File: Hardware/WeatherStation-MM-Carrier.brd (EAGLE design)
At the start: 67.3 x 58.4 mm, 156 parts, among them J11 microSD, J13 RJ11 - WIND, J15 MICROMOD-2222-C, J2 JTAG, J3 QWIIC_RIGHT_ANGLE, J7 RJ11 - RAIN, U1 BME280, U2 VEML6075, U3 AS3935, U5 AP7361C-33FGEUDFN-8

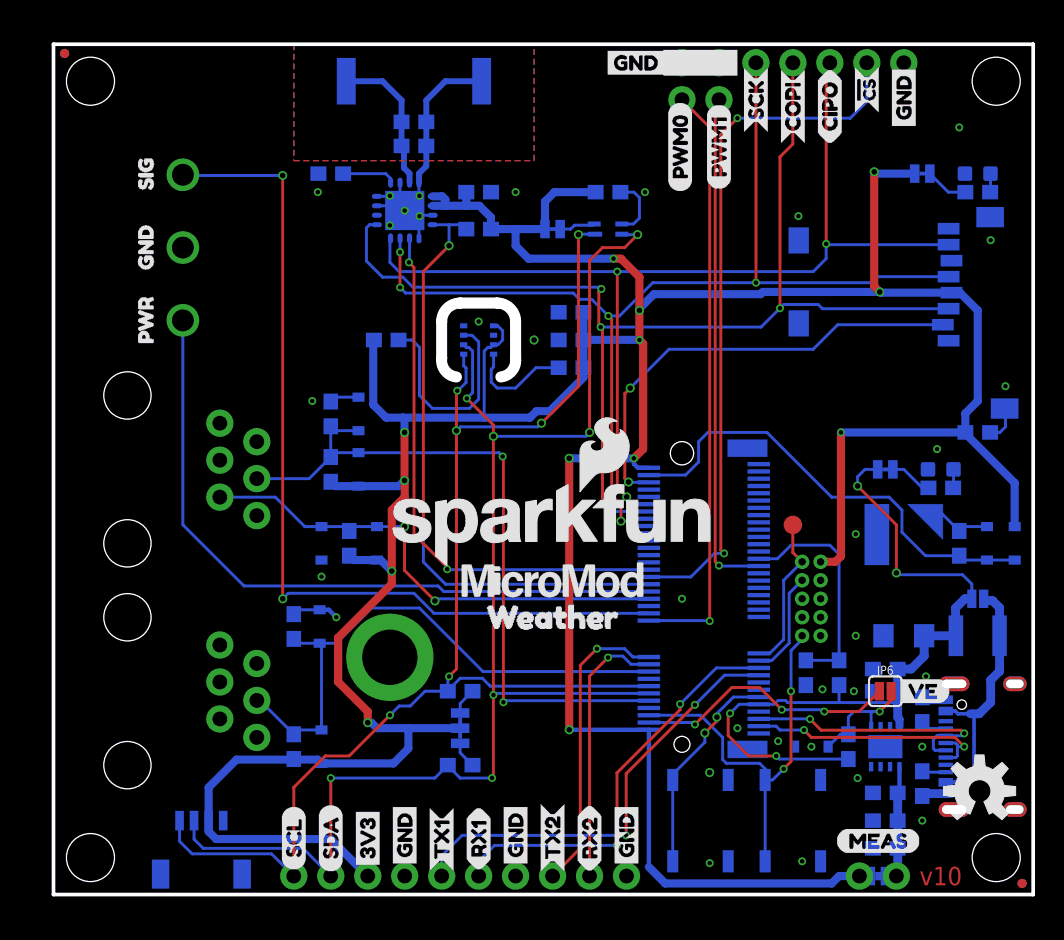
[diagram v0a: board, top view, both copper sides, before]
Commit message: Update WeatherStation-MM-Carrier.brd
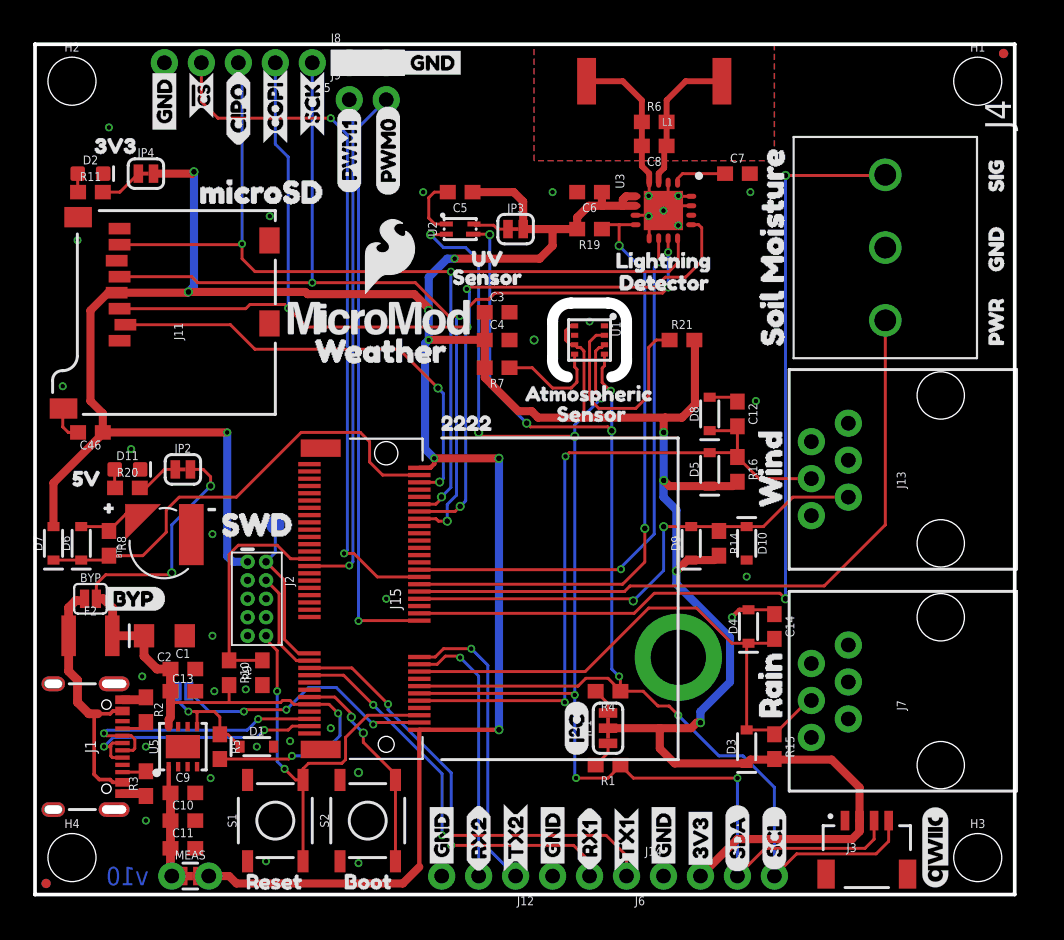
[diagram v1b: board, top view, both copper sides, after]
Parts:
- moved FD1 67.1 mm to (0.76, 0.76), flipped to the top
- moved FD3 67.1 mm to (0.76, 0.76), flipped to the bottom
- moved D7 66.0 mm to (1.27, 24.1), flipped to the top
- moved U$18 65.3 mm to (1.65, 28.6), flipped to the top
- moved FD2 64.5 mm to (66.5, 57.8), flipped to the top
- moved FD4 64.5 mm to (66.5, 57.8), flipped to the bottom
- moved H2 63.5 mm to (2.54, 55.9), flipped to the top
- moved H4 63.5 mm to (2.54, 2.54), flipped to the top
- moved U$12 63.5 mm to (66.0, 36.8), flipped to the top
- moved U$13 63.5 mm to (66.0, 47.4), flipped to the top
- moved U$4 63.5 mm to (66.0, 41.9), flipped to the top
- moved D6 62.2 mm to (3.17, 24.1), flipped to the top
- moved U$1 62.2 mm to (3.17, 51.4), flipped to the top
- moved LOGO3 61.2 mm to (3.68, 7.11), flipped to the bottom
- moved BYP 61.0 mm to (3.81, 20.3), flipped to the top
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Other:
- outline, holes or cut-outs redrawn
